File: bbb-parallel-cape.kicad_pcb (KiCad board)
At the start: 2 copper layers, 54.6 x 86.4 mm, 45 parts, among them IC201 GTL2003PW, IC202 GTL2003PW, IC203 GTL2003PW, IC204 GTL2003PW, IC205 GTL2003PW, P101 IDC26, P102 BeagleBone_Black_Header, P103 BeagleBone_Black_Header, P104 IDC26, P105 Conn_02x03_Odd_Even, Q101 2N7002K, SW101 SW_Push, SW102 SW_Push

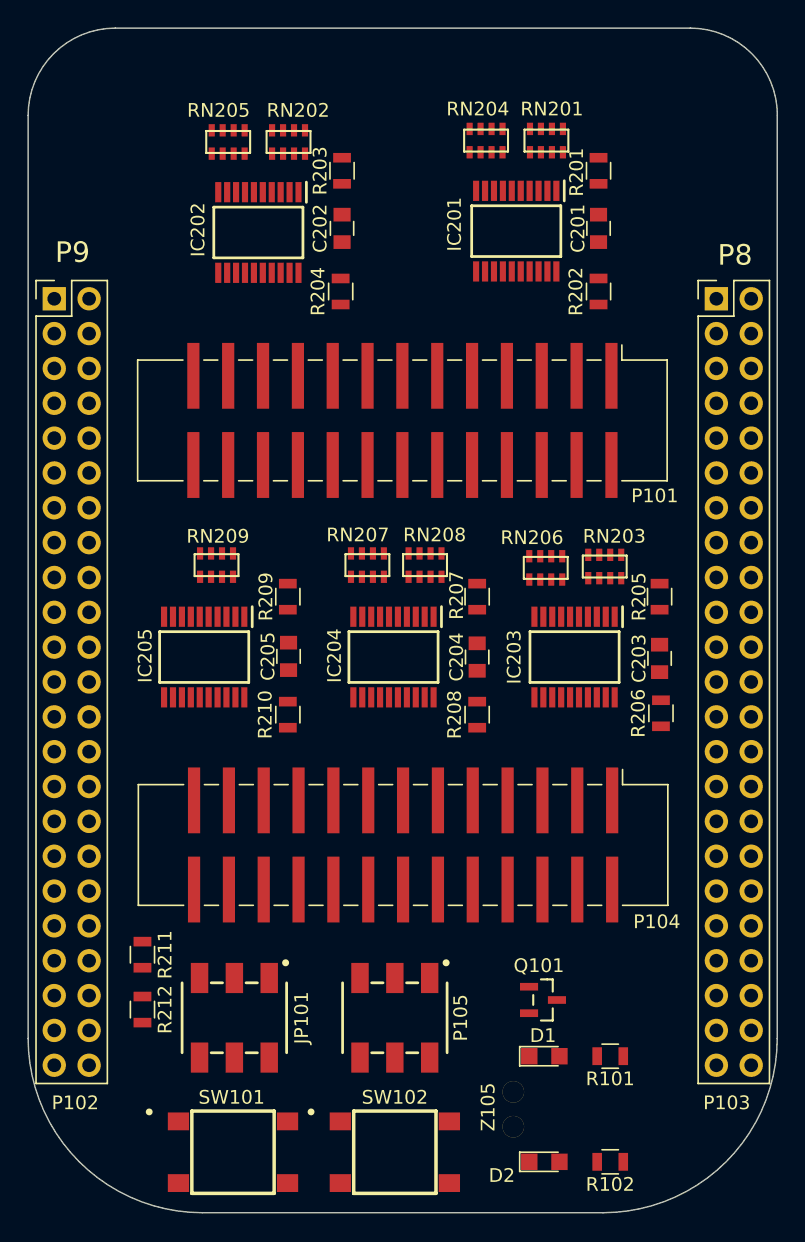
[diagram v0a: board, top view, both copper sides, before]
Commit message: revision1 files
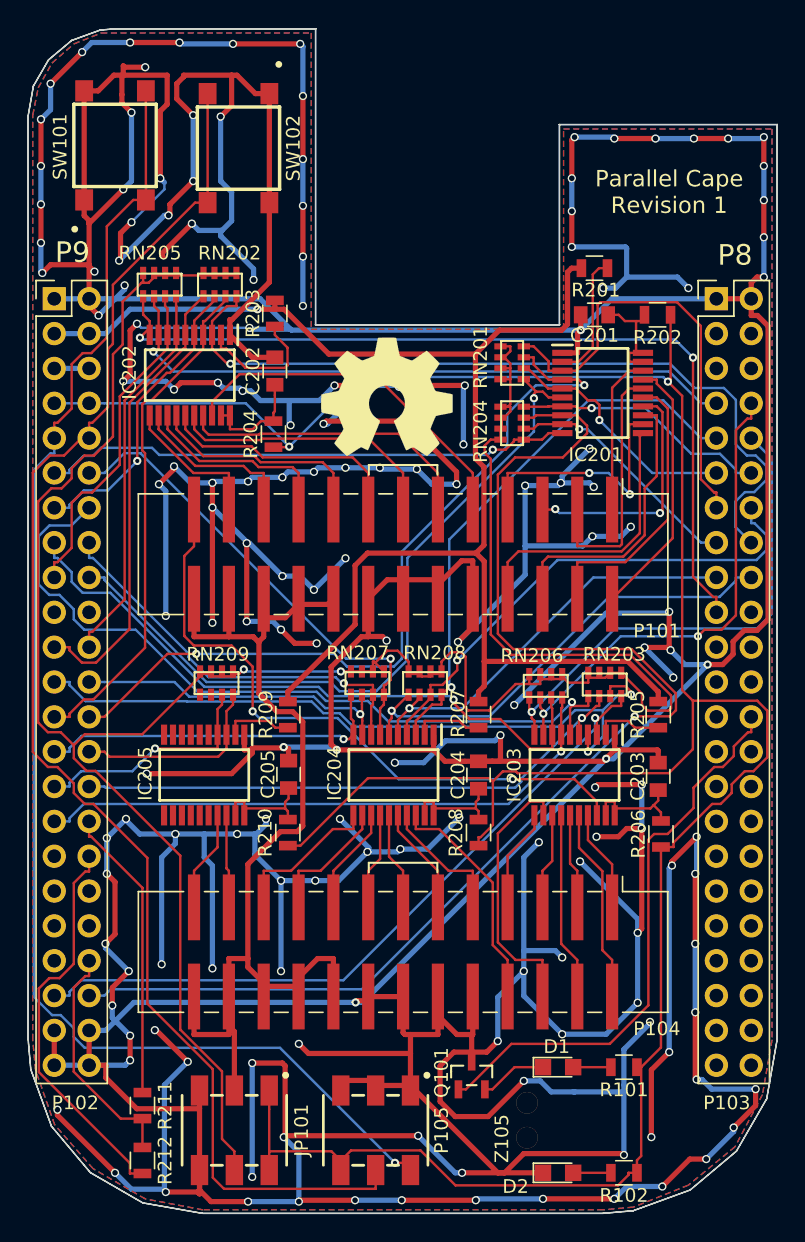
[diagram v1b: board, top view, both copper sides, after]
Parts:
- added G***: LOGO, footprint:OSHW, F.Cu at (140.6, 69.6)
- moved SW102 74.1 mm to (129.8, 51.4), turned to 270 degrees
- moved SW101 73.9 mm to (120.8, 51.2), turned to 90 degrees
- moved RN204 20.7 mm to (149.8, 71.5), turned to 270 degrees
- moved RN201 16.4 mm to (149.8, 67.0), turned to 270 degrees
- moved IC201 13.4 mm to (156.3, 69.2), turned to 0 degrees
- moved IC202 11.5 mm to (126.2, 68.0)
- moved RN205 11.5 mm to (124.0, 61.4)
- moved RN202 11.5 mm to (128.4, 61.4)
- moved C202 11.5 mm to (132.4, 67.7)
- moved R203 11.5 mm to (132.4, 63.5)
- moved R204 11.5 mm to (132.3, 72.2)
- moved R211 11.0 mm to (122.8, 121.2)
- moved R212 11.0 mm to (122.8, 125.2)
- moved P101 9.75 mm to (141.8, 81.0)
- moved R206 8.80 mm to (160.6, 101.4)
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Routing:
- net GNDD: track 0.00 -> 1074.0 mm, vias 0 -> 166
- net SYS_5V: track 0.00 -> 200.2 mm, vias 0 -> 2
- net PU_OR_PD: track 0.00 -> 189.3 mm, vias 0 -> 2
- net +3V3: track 0.00 -> 107.7 mm, vias 0 -> 1
- net SYS_RESETn: track 0.00 -> 105.9 mm
- net PWR_BUT: track 0.00 -> 103.7 mm, vias 0 -> 1
- net IO5_BB: track 0.00 -> 92.3 mm, vias 0 -> 1
- net GND_OR_5V: track 0.00 -> 77.4 mm
- net IO15_BB: track 0.00 -> 64.3 mm, vias 0 -> 2
- net IO1_BB: track 0.00 -> 58.4 mm, vias 0 -> 2
- net IO8_BB: track 0.00 -> 58.2 mm, vias 0 -> 1
- net IO19_BB: track 0.00 -> 56.4 mm, vias 0 -> 1
- net IO3_BB: track 0.00 -> 54.5 mm, vias 0 -> 1
- net IO16_BB: track 0.00 -> 52.6 mm, vias 0 -> 1
- net IO17_BB: track 0.00 -> 51.8 mm, vias 0 -> 2
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- added copper zone on B.Cu, net GNDD
- added copper zone on F.Cu, net GNDD
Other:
- outline, holes or cut-outs redrawn
- board text added: "Parallel Cape Revision 1"
